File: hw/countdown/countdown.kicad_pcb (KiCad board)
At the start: 4 copper layers, 44 x 23 mm, 24 parts, among them J1 TC2030-SWD, SW1 TS-1187A-B-A-B, U1 STM32L031G6U6, Y1 32.768kHz

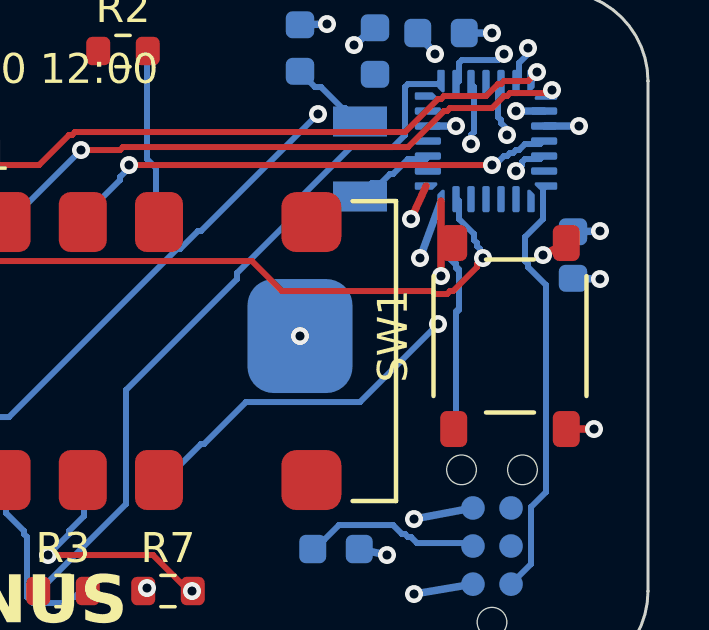
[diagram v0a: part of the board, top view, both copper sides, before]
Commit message: Design log: routing endgame narrative
Co-Authored-By: Claude Fable 5 <noreply@anthropic.com>
Claude-Session: https://claude.ai/code/session_01EyK7WVGPpPEnSjWLWWV8on
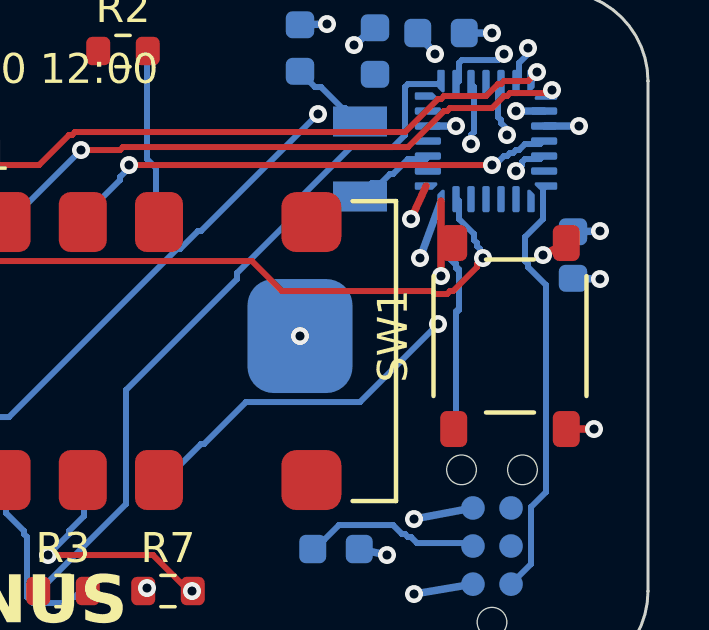
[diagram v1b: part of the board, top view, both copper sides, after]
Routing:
- net GND: track 166.2 -> 182.1 mm

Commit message: Prompt log updates
Co-Authored-By: Claude Fable 5 <noreply@anthropic.com>
Claude-Session: https://claude.ai/code/session_01EyK7WVGPpPEnSjWLWWV8on
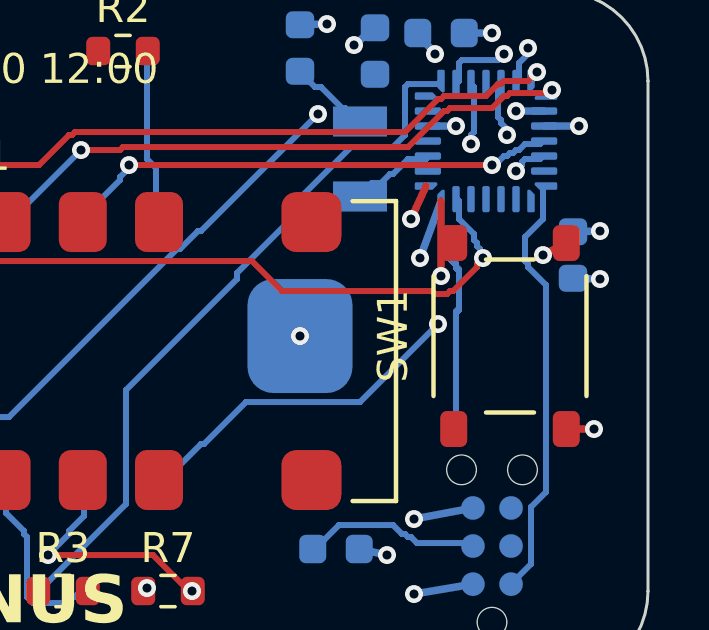
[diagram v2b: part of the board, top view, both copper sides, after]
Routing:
- net GND: track 182.1 -> 213.9 mm
